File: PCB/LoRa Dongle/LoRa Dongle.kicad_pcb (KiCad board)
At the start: 4 copper layers, 22.5 x 36.5 mm, 47 parts, among them IC1 BALFHB-WL-06D3, J1 Conn_01x04_Socket, J2 USB_C_Receptacle_USB2.0_16P, J3 Header_01x05, U1 USBLC6-2SC6, U2 CP2102N-Axx-xQFN28, U3 AP2112K-3.3, U4 STM32WLE5CCUx, U5 BGS12WN6E6327, U6 RFPC-SMA27, Y1 Crystal

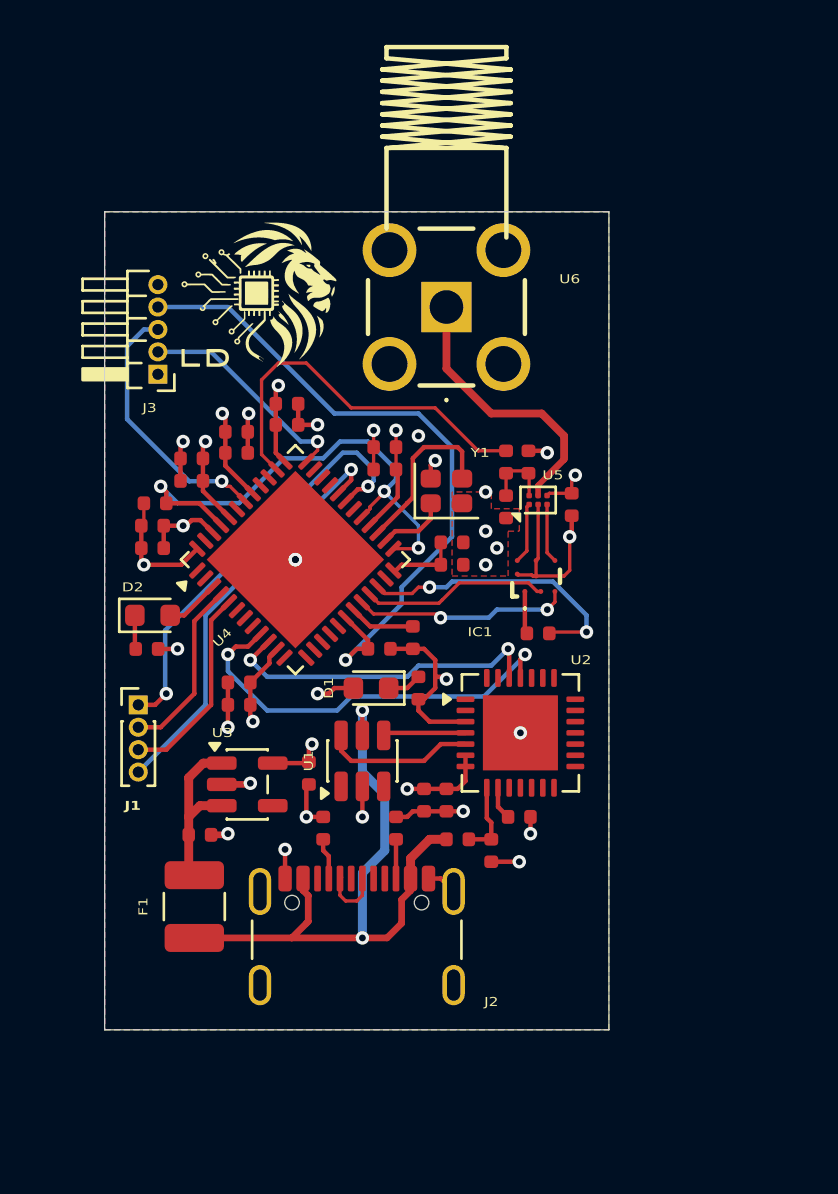
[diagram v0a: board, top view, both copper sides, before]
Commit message: second try- layout
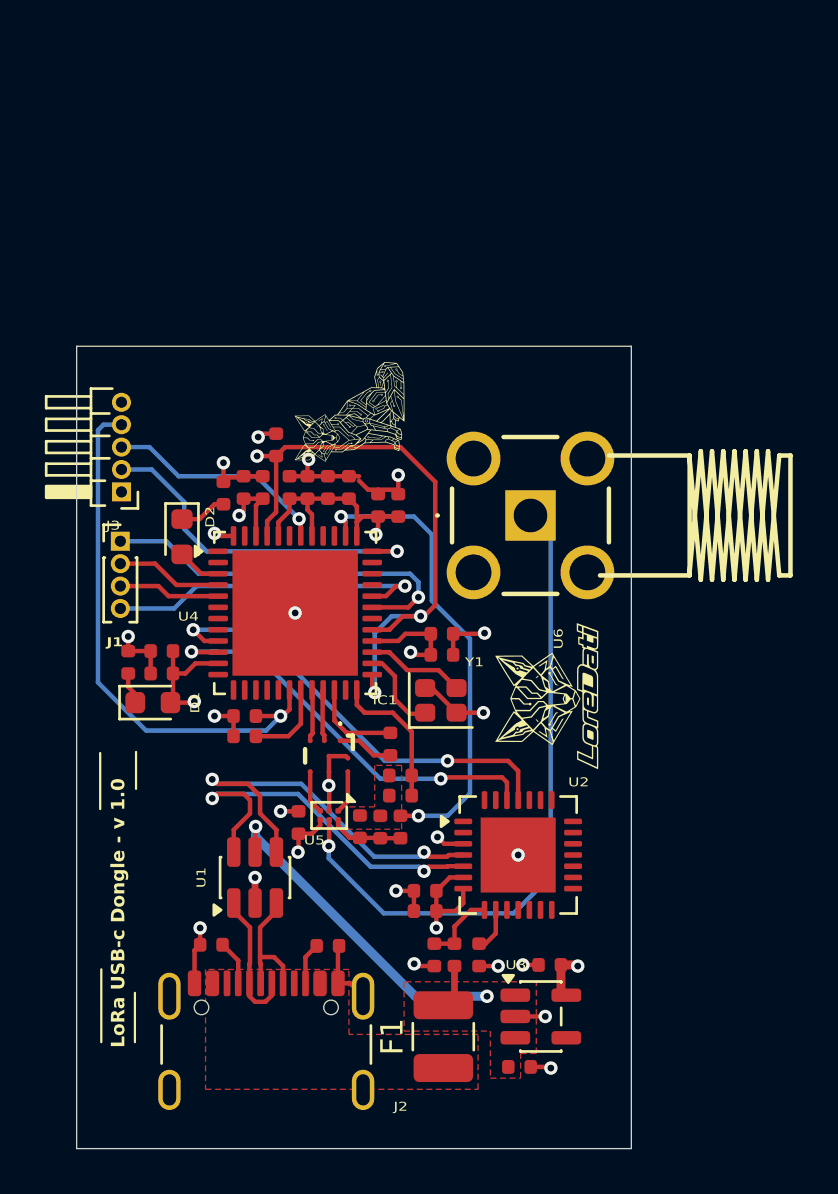
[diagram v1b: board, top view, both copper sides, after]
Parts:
- moved C25 18.7 mm to (54.1, 116.2), turned to 90 degrees
- moved C6 17.6 mm to (64.0, 127.2)
- moved C21 17.6 mm to (57.8, 116.5)
- moved R8 17.0 mm to (58.7, 116.5)
- moved U5 16.9 mm to (55.5, 115.9), turned to -90 degrees
- moved U3 16.7 mm to (65.0, 124.9)
- moved C20 15.7 mm to (56.9, 116.4), turned to 90 degrees
- moved C5 13.7 mm to (65.4, 122.6), turned to 180 degrees
- moved R9 13.0 mm to (46.5, 109.1), turned to 90 degrees
- moved F1 12.5 mm to (60.6, 125.8)
- moved C26 12.4 mm to (60.5, 107.8)
- moved C27 12.4 mm to (60.5, 108.8)
- moved IC1 12.2 mm to (55.5, 113.3), turned to -90 degrees
- moved C8 11.5 mm to (58.7, 115.0), turned to 180 degrees
- moved U6 10.0 mm to (64.5, 102.5), turned to 180 degrees
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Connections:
- net Net-(J2-D+-PadA6) renamed /Connectors/USB_D+
- net Net-(J2-D--PadA7) renamed /Connectors/USB_D-
- net Net-(U2-D+) renamed /Connectors/ESD_D+
- net Net-(U2-D-) renamed /Connectors/ESD_D-
- C6 pad 1: /MCU/5V -> VBUS
- F1 pad 1: VBUS -> VBUS_IN
- F1 pad 2: /MCU/5V -> VBUS
- J2 pad A4: VBUS -> VBUS_IN
- J2 pad A9: VBUS -> VBUS_IN
- J2 pad B4: VBUS -> VBUS_IN
- J2 pad B9: VBUS -> VBUS_IN
- R6 pad 1: +3V3 -> Net-(U2-~{RST})
- R6 pad 2: Net-(U2-~{RST}) -> +3V3
- U3 pad 1: /MCU/5V -> VBUS
- U3 pad 3: /MCU/5V -> VBUS
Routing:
- net RF_OUT: track 12.4 -> 29.8 mm, vias 0 -> 1
- net /Connectors/ESD_D+: track 3.70 -> 18.1 mm, vias 0 -> 2
- net VBUS: track 29.7 -> 16.8 mm
- net /Connectors/ESD_D-: track 6.73 -> 17.3 mm, vias 0 -> 2
- net RFO_LP: track 12.8 -> 4.09 mm, vias 2 -> 0
- net /MCU/5V: track 7.88 -> 0.00 mm
- net GND: track 45.9 -> 38.2 mm, vias 26 -> 21
- net RFI_P: track 9.67 -> 2.32 mm, vias 2 -> 0
- net RFI_N: track 8.34 -> 2.30 mm
- net NRST: track 30.2 -> 24.2 mm
- net /Connectors/USB_D+: track 0.01 -> 5.85 mm
- net SWDIO: track 9.89 -> 15.6 mm
- net SDA: track 8.99 -> 4.55 mm
- net RF_CTRL: track 17.1 -> 21.2 mm, vias 0 -> 2
- net GPIO_2: track 18.7 -> 14.8 mm
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- added copper zone on F.Cu, net VBUS
- added copper zone on F.Cu, net VBUS_IN
- removed copper zone on B.Cu, net GND
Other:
- board size 22.5 x 36.5 mm -> 24.8 x 35.8 mm
- board text added: "LoRa USB-c Dongle - v 1.0"

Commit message: Use shared Kicad_Libs instead of project-specific libraries
- Project parts moved to Kicad_Libs (symbol, footprint, 3D, datasheet)
- Lib tables point to ${KIPRJMOD}/../KiCad_Libs (link via bring_libs.bat)
- Schematic/PCB references (lib ids, footprints, 3D paths, datasheets)
  updated to the Kicad_Libs libraries; no design changes
- Removed the old project-specific library folder
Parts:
- IC1: footprint BALFHB-WL-06D3:BALFHBWL06D3 -> eRFModule:BALFHBWL06D3
- U6: footprint RFPC-SMA27-F:RFPCSMA27F -> eConnector:RFPCSMA27F
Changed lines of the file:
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@@
 		)
 	)
-	(footprint "BALFHB-WL-06D3:BALFHBWL06D3"
+	(footprint "eRFModule:BALFHBWL06D3"
 		(layer "F.Cu")
 		(at 55.51 113.29 -90)
@@
 		)
 		(embedded_fonts no)
-		(model "BALFHB-WL-06D3.stp"
+		(model "${KIPRJMOD}/../KiCad_Libs/eRFModule/eRFModule.3dshapes/BALFHB-WL-06D3.stp"
 			(offset
 				(xyz 0 0 0)
@@
 		)
 	)
-	(footprint "RFPC-SMA27-F:RFPCSMA27F"
+	(footprint "eConnector:RFPCSMA27F"
 		(layer "F.Cu")
 		(at 64.5 102.55 180)
@@
 		)
 		(embedded_fonts no)
-		(model "RFPC-SMA27-F.stp"
+		(model "${KIPRJMOD}/../KiCad_Libs/eConnector/eConnector.3dshapes/RFPC-SMA27-F.stp"
 			(offset
 				(xyz -0.05 0 0.28)
@@
 		)
 		(embedded_fonts no)
-		(model "C:/Users/lollo/Desktop/Hardware_Projects/LoRa/Library/BGS12WN6E6327XTSA1/BGS12WN6E6327XTSA1.stp"
+		(model "${KIPRJMOD}/../KiCad_Libs/eRFModule/eRFModule.3dshapes/BGS12WN6E6327XTSA1.stp"
 			(offset
 				(xyz 0 0 0)
